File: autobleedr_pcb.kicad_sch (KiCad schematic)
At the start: 25 parts, among them J1 Barrel_Jack, J10 XT60 Connector, J11 Conn_01x02_Pin, J13 Screw_Terminal_01x08, J2 Conn_01x01_Pin, J4 Conn_01x13_Pin, J5 Conn_01x13_Pin, J7 Screw_Terminal_01x02, J8 Conn_01x02_Pin, J9 Conn_01x02_Pin, U2 ESP32, U4 Buck Converter, U6 TMC2209

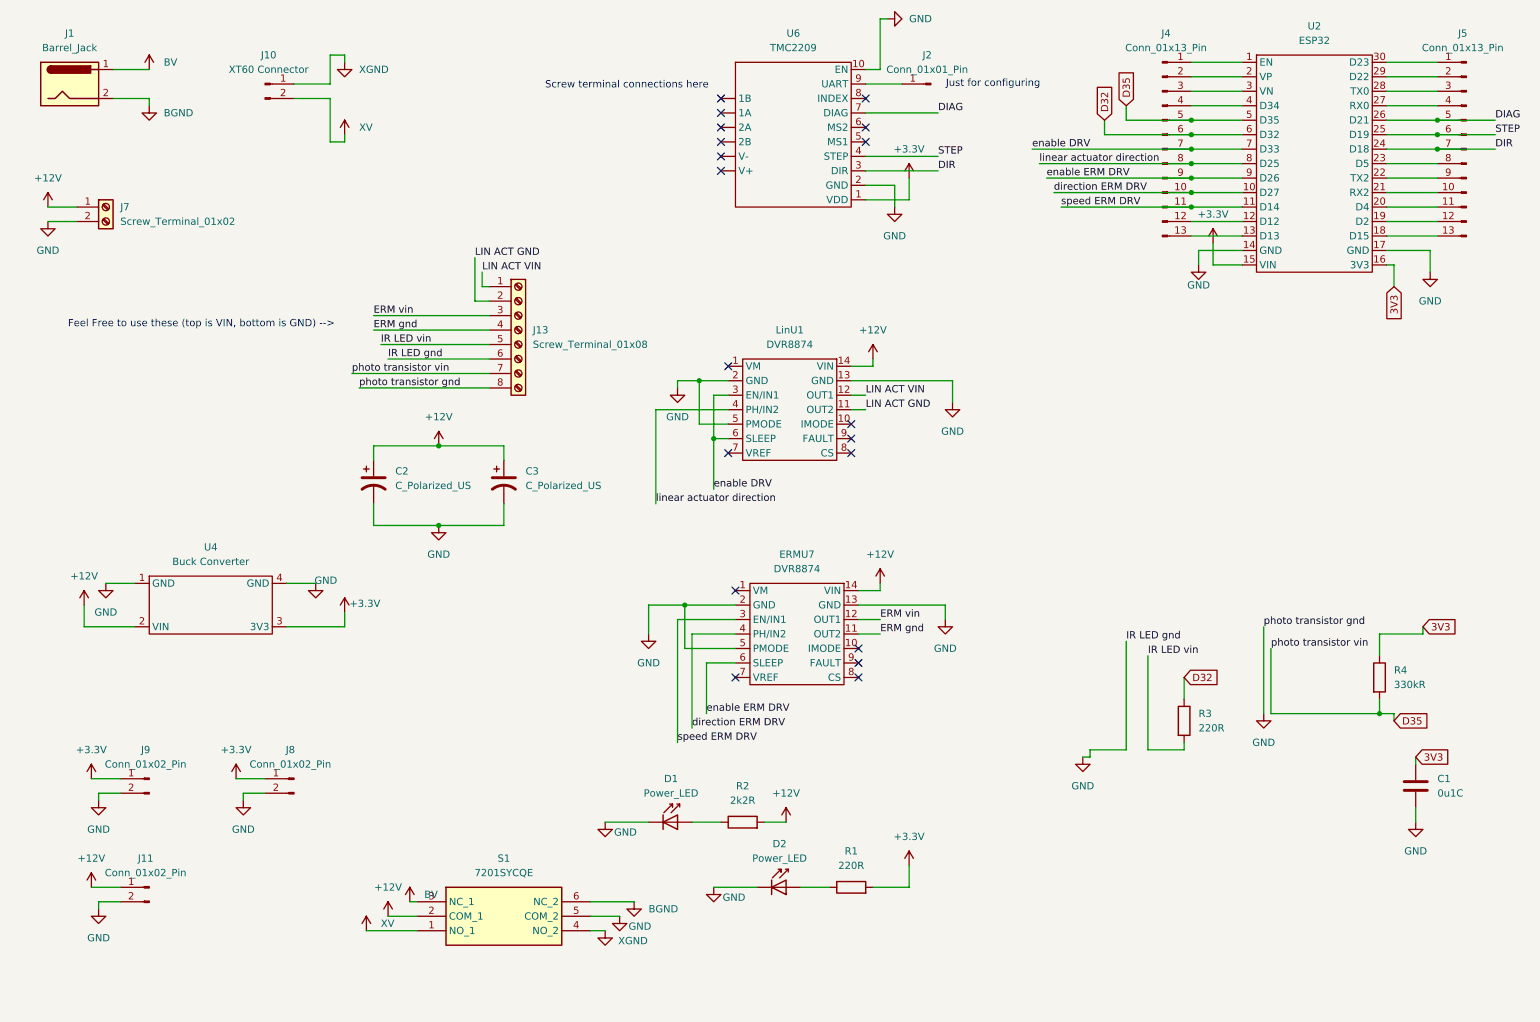
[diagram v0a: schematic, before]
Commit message: Made some changes for Barnes
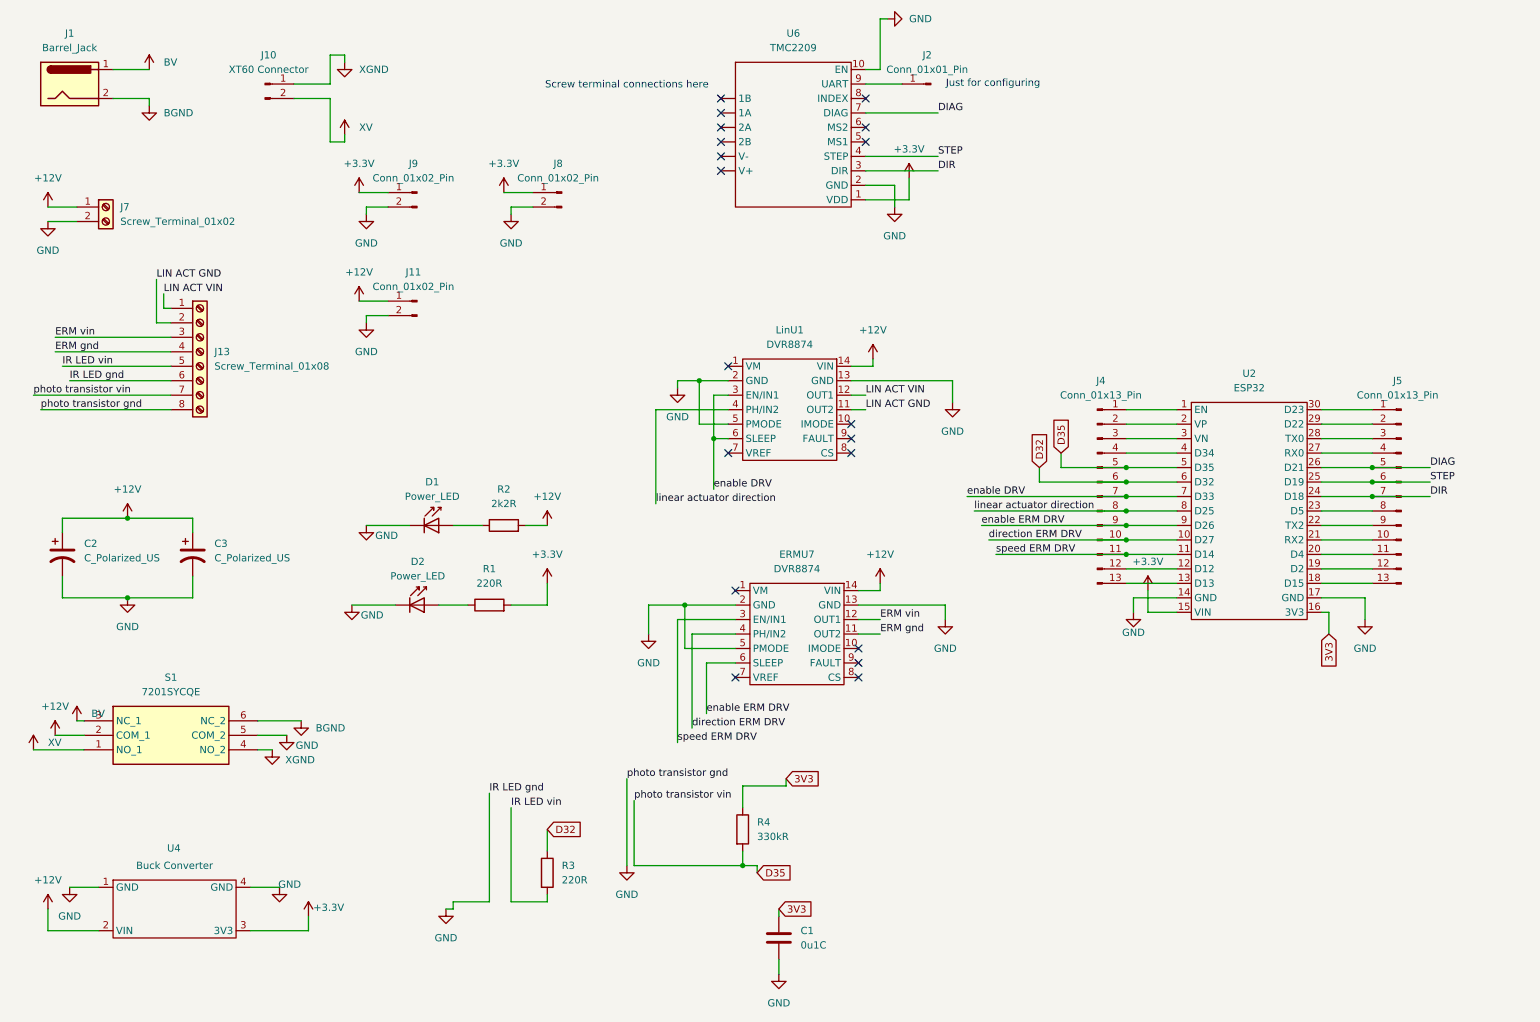
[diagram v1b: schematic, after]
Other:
- note removed: "Feel Free to use these (top is VIN, bottom is GND) -->"
- moved on the sheet: C1, C2, C3, D1, D2, J11, J13, J4, J5, J8, J9, R1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
